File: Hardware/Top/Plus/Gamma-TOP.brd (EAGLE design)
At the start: 38 x 38 mm, 63 parts, among them SW1 SWITCH.MOM, SW2 SWITCH.MOM, U1 FT231XS, U3 NRF52832_MODULE_MDBT42, U5 FT24C64A, Y1 32.768kHz

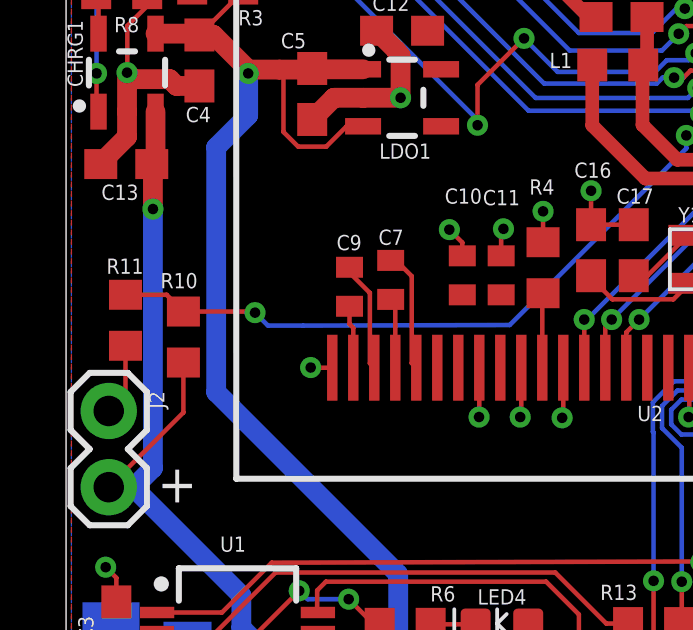
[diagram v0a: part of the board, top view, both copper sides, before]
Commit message: small fixes
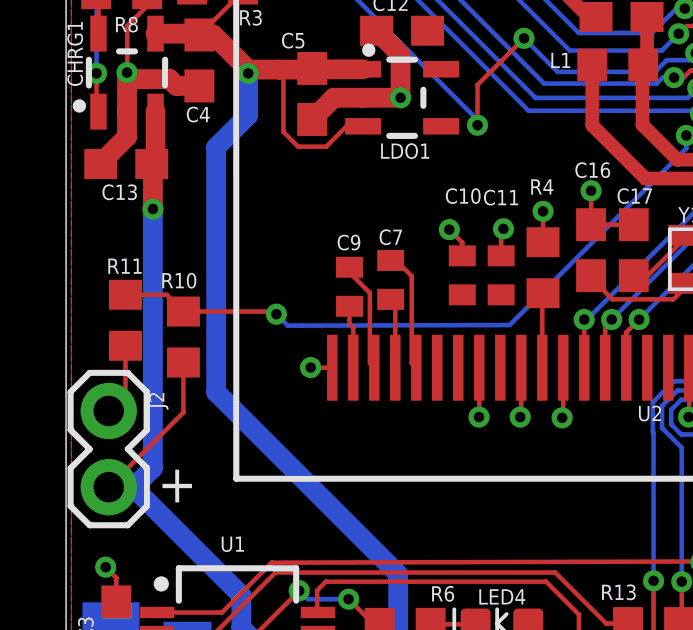
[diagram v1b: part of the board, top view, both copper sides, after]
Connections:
- net GND: no longer SW1.B2, SW2.B2
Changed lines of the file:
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@@
 <?xml version="1.0" encoding="utf-8"?>
 <!DOCTYPE eagle SYSTEM "eagle.dtd">
-<eagle version="9.5.2">
+<eagle version="9.6.2">
 <drawing>
 <settings>
@@
 <contactref element="R11" pad="1"/>
 <contactref element="CHRG1" pad="2"/>
-<contactref element="SW1" pad="B2"/>
 <contactref element="SW1" pad="B1"/>
 <contactref element="SW2" pad="B1"/>
-<contactref element="SW2" pad="B2"/>
 <contactref element="JP1" pad="1"/>
 <contactref element="C3" pad="1"/>
@@
 <contactref element="C18" pad="2"/>
 <contactref element="C21" pad="2"/>
-<wire x1="25.9714" y1="1.6616" x2="28.1814" y2="1.7124" width="0" layer="19" extent="1-1"/>
-<wire x1="18.0214" y1="1.6616" x2="16.3576" y2="4.572" width="0" layer="19" extent="1-1"/>
 </signal>
 <signal name="SWDIO">
@@
 <wire x1="20.6756" y1="25.9228" x2="14.788509375" y2="20.035709375" width="0.1524" layer="16"/>
 <wire x1="14.788509375" y1="20.035709375" x2="7.8994" y2="20.015046875" width="0.1524" layer="16"/>
-<via x="6.2992" y="20.447" extent="1-16" drill="0.35"/>
+<via x="7.0104" y="20.3962" extent="1-16" drill="0.35"/>
 <wire x1="22.4764" y1="26.318" x2="20.7122" y2="26.318" width="0.1524" layer="1"/>
 <wire x1="20.7122" y1="26.318" x2="20.6756" y2="26.3546" width="0.1524" layer="1"/>
 <wire x1="3.3528" y1="21.043" x2="3.9116" y2="20.4842" width="0.1524" layer="1"/>
-<wire x1="6.262" y1="20.4842" x2="6.2992" y2="20.447" width="0.1524" layer="1"/>
-<wire x1="3.9116" y1="20.4842" x2="6.262" y2="20.4842" width="0.1524" layer="1"/>
-<wire x1="7.8994" y1="20.015046875" x2="6.731153125" y2="20.015046875" width="0.1524" layer="16"/>
-<wire x1="6.731153125" y1="20.015046875" x2="6.2992" y2="20.447" width="0.1524" layer="16"/>
+<wire x1="6.9224" y1="20.4842" x2="7.0104" y2="20.3962" width="0.1524" layer="1"/>
+<wire x1="3.9116" y1="20.4842" x2="6.9224" y2="20.4842" width="0.1524" layer="1"/>
+<wire x1="7.8994" y1="20.015046875" x2="7.391553125" y2="20.015046875" width="0.1524" layer="16"/>
+<wire x1="7.391553125" y1="20.015046875" x2="7.0104" y2="20.3962" width="0.1524" layer="16"/>
 </signal>
 <signal name="D30/LED.CTRL">
